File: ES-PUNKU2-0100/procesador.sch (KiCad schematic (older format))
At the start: 33 parts, among them J1 PROGRAMACION, J2 12VDC, J3 BOOT, J4 Micro_SD_Card, SW1 RESET, U1 LM2575S5, U2 ESP32-WROOM-32D, U3 LD1117S33, U4 MCP7940N, Y1 32,768KHz

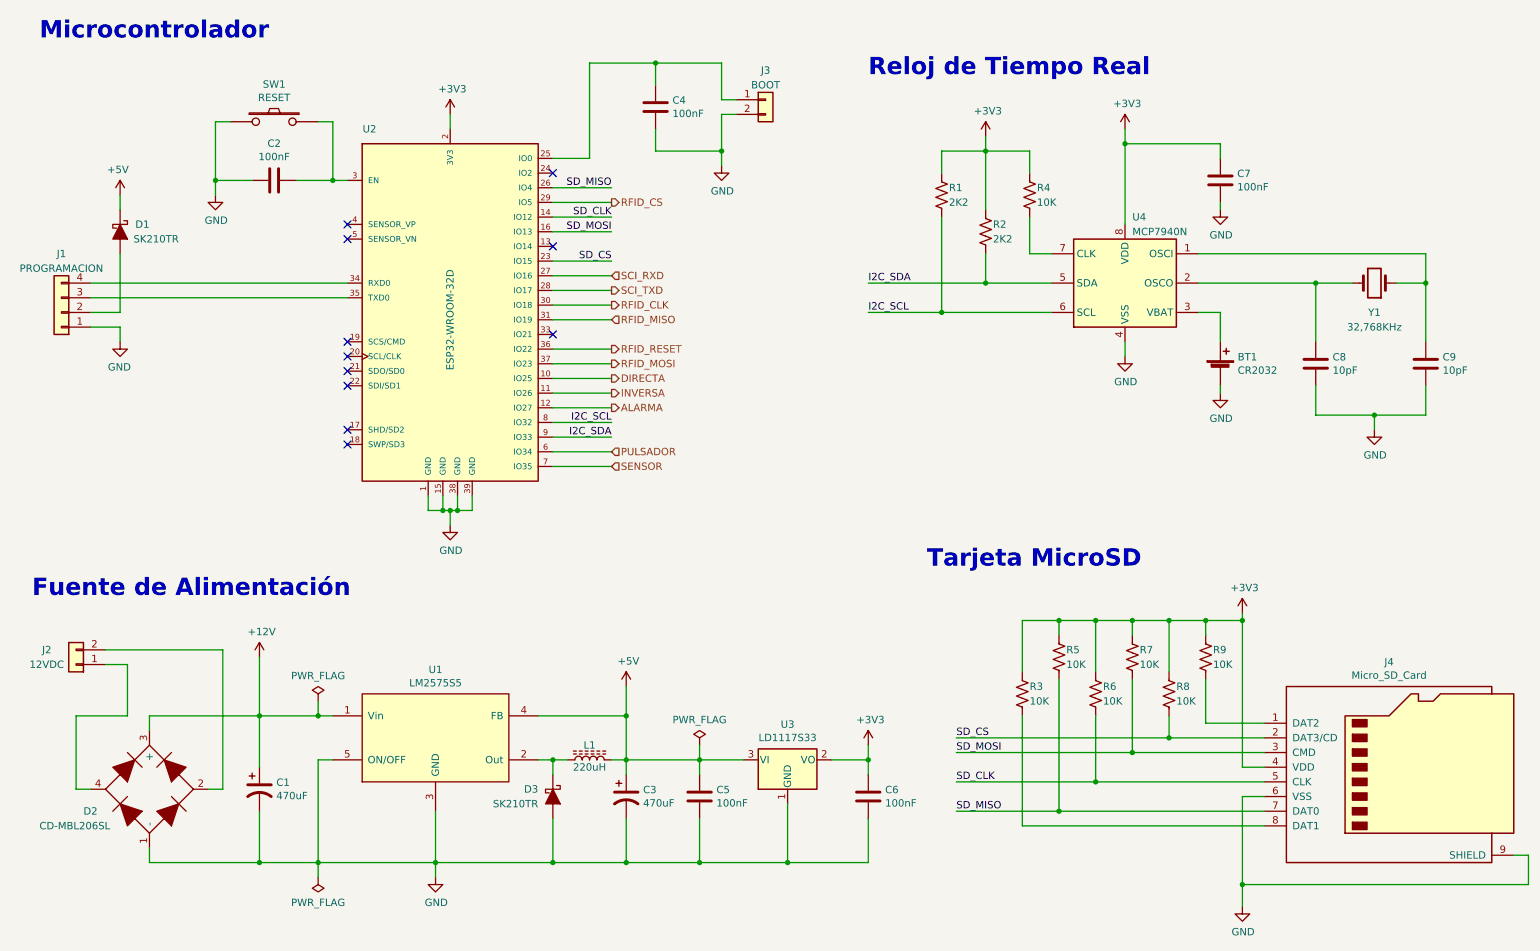
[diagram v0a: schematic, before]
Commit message: Primera versión ruteada de la placa
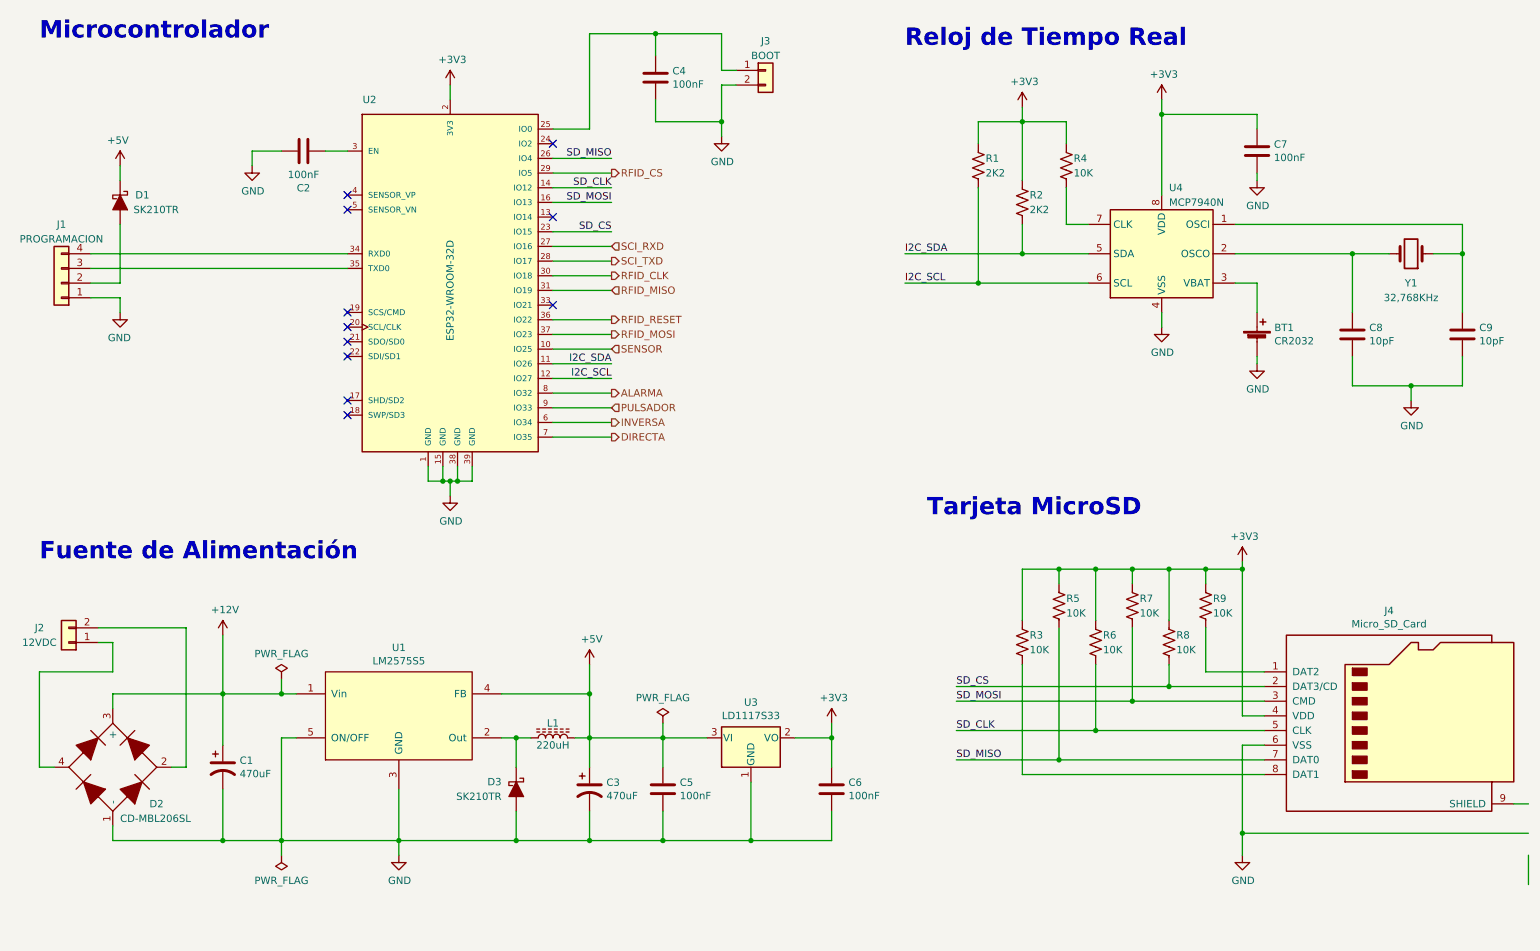
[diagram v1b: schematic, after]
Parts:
- removed SW1: RESET, encapsulados:TACT_SWITCH, symbol componentes:SW_PUSH
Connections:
- net ALARMA: now also U2.8 (IO32); no longer U2.12 (IO27)
- net DIRECTA: now also U2.7 (IO35); no longer U2.10 (IO25)
- net GND: now also C2.1; no longer C2.2, J4.9 (SHIELD)
- net I2C_SCL: now also U2.12 (IO27); no longer U2.8 (IO32)
- net I2C_SDA: now also U2.11 (IO26); no longer U2.9 (IO33)
- net INVERSA: now also U2.6 (IO34); no longer U2.11 (IO26)
- net PULSADOR: now also U2.9 (IO33); no longer U2.6 (IO34)
- net SENSOR: now also U2.10 (IO25); no longer U2.7 (IO35)
- net at U2.3 (EN): now also C2.2; no longer C2.1
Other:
- moved on the sheet: BT1, C1, C2, C3, C4, C5, C6, C7, C8, C9, D1, D2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
